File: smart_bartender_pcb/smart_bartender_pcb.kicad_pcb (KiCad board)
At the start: 2 copper layers, 103.4 x 104.7 mm, 48 parts, among them J1 Screw_Terminal_01x02, U1 AMS1117-5.0, U2 ULN2803A

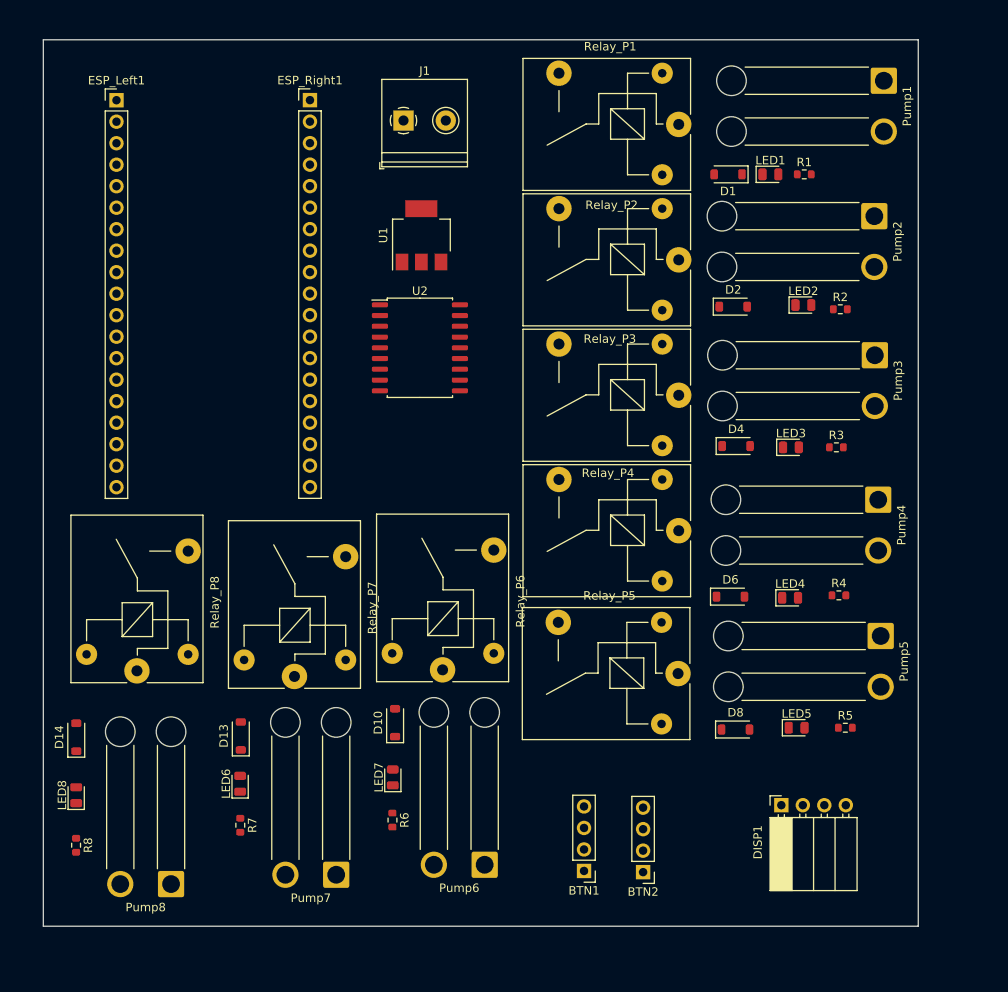
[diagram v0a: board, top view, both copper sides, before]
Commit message: updated pcb
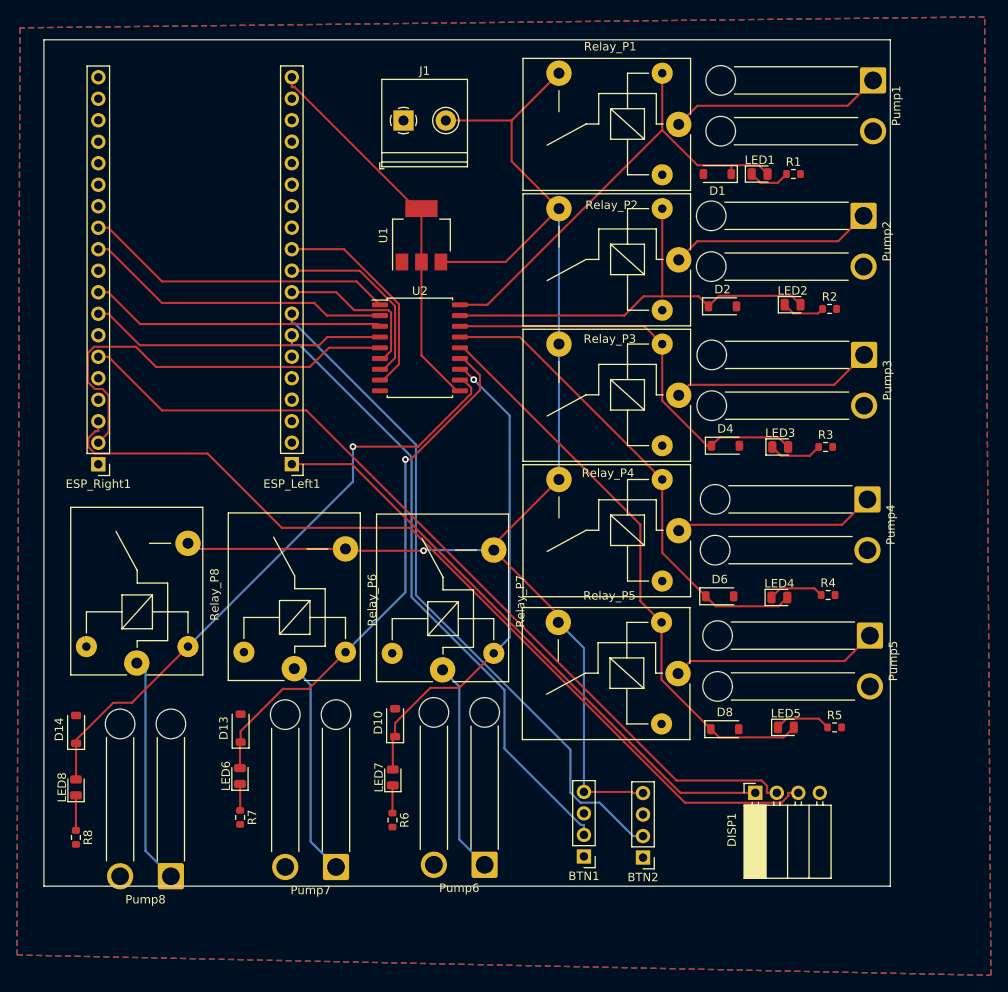
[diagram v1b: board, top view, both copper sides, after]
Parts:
- moved ESP_Left1 3.46 mm to (47.9, 47.3), turned to 180 degrees
- moved ESP_Right1 3.46 mm to (47.9, 47.3), turned to 180 degrees
- moved DISP1 3.40 mm to (114.0, 109.0)
- moved BTN1 1.72 mm to (93.8, 116.5)
- moved BTN2 1.72 mm to (100.8, 116.6)
- moved Pump2 1.27 mm to (126.8, 40.8)
- moved R2 1.27 mm to (122.8, 51.8)
- moved D8 1.27 mm to (110.4, 101.5)
- moved Pump5 1.27 mm to (127.6, 90.4)
- moved D4 1.27 mm to (110.5, 68.0)
- moved D6 1.27 mm to (109.8, 85.8)
- moved LED2 1.27 mm to (118.5, 51.3)
- moved LED3 1.27 mm to (117.0, 68.1)
- moved LED4 1.27 mm to (116.9, 85.9)
- moved LED5 1.27 mm to (117.7, 101.2)
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- renumbered Relay_P7 to Relay_P6, Relay_P6 to Relay_P7
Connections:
- DISP1 pad 1: unconnected-(DISP1-3V3-Pad1) -> 3V3
- DISP1 pad 2: unconnected-(DISP1-SDA-Pad2) -> SDA
- DISP1 pad 3: unconnected-(DISP1-SCL-Pad3) -> SCL
- DISP1 pad 4: unconnected-(DISP1-GND-Pad4) -> GND
- ESP_Left1 pad 1: unconnected-(ESP_Left1-3V3-Pad1) -> 3V3
- ESP_Left1 pad 10: BTN1 -> P7
- ESP_Left1 pad 11: BTN2 -> P8
- ESP_Left1 pad 7: unconnected-(ESP_Left1-P32-Pad7) -> BTN1
- ESP_Left1 pad 8: unconnected-(ESP_Left1-P33-Pad8) -> BTN2
- ESP_Left1 pad 9: P8 -> P6
- ESP_Right1 pad 33: P5 -> SDA
- ESP_Right1 pad 36: P6 -> SCL
- ESP_Right1 pad 37: P7 -> P5
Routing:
- net 12V: track 0.00 -> 165.0 mm, vias 0 -> 1
- net SCL: track 0.00 -> 105.7 mm
- net SDA: track 0.00 -> 102.0 mm
- net BTN2: track 0.00 -> 81.1 mm
- net BTN1: track 0.00 -> 74.1 mm
- net 5V_P8: track 0.00 -> 73.1 mm, vias 0 -> 1
- net 3V3: track 0.00 -> 70.8 mm
- net 5V_P5: track 0.00 -> 68.3 mm
- net 5V_P6: track 0.00 -> 63.5 mm, vias 0 -> 1
- net 5V_P7: track 0.00 -> 57.7 mm, vias 0 -> 1
- net 5V_P4: track 0.00 -> 57.4 mm
- net 5V_P1: track 0.00 -> 54.8 mm
- net 5V_P2: track 0.00 -> 53.0 mm
- net 5V_P3: track 0.00 -> 49.4 mm
- net P5: track 0.00 -> 49.4 mm
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- added copper zone on B.Cu, net GND
- added copper zone on F.Cu, net GND
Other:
- board size 103.4 x 104.7 mm -> 100 x 100 mm
